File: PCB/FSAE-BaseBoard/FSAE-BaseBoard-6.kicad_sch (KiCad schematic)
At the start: 9 parts, among them J5 Conn_01x02, J6 Conn_01x03, J7 Conn_01x02, U9 SN65HVD230

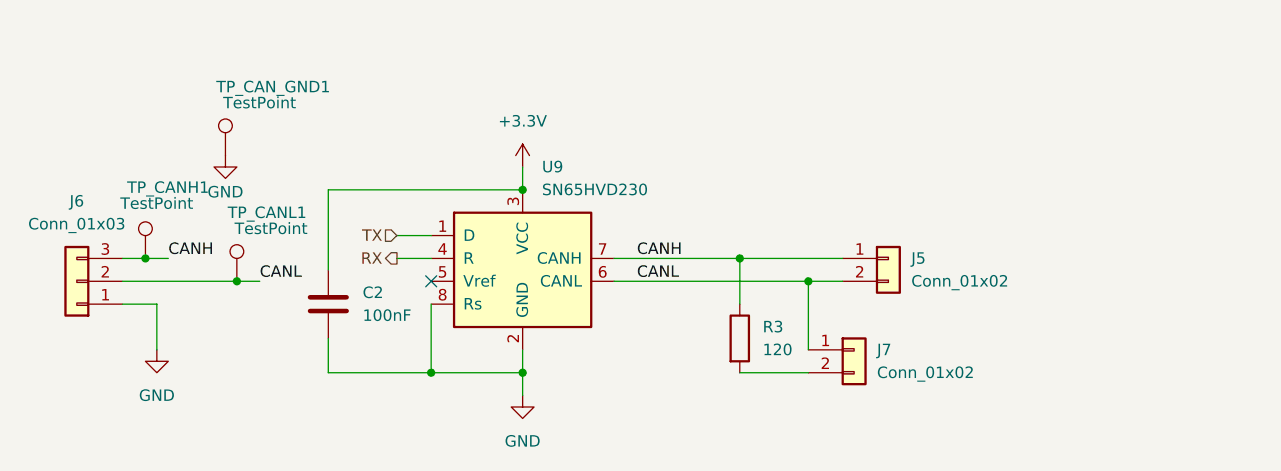
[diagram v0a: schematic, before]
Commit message: Actualizacion de la placa de desarollo - v.2
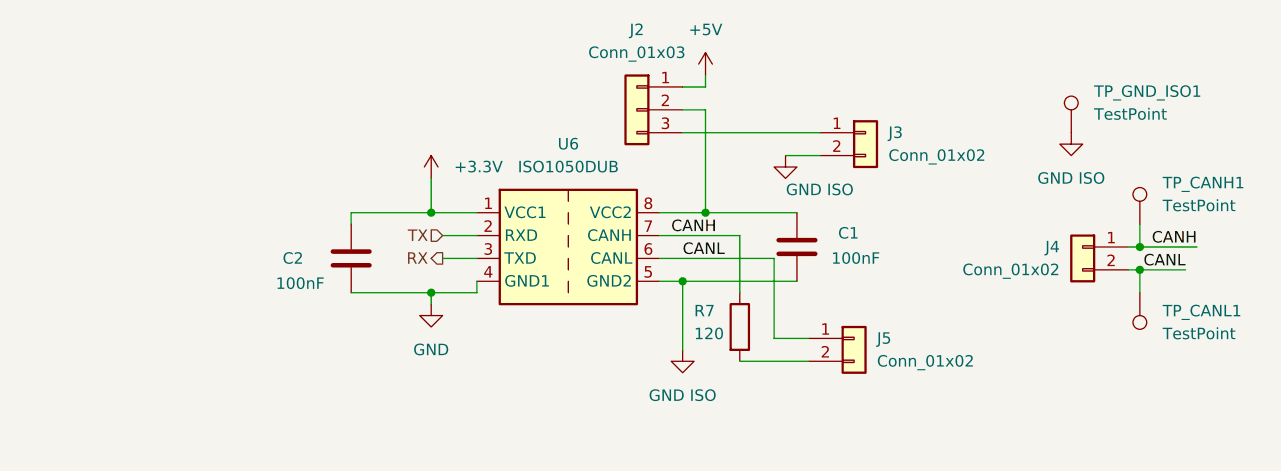
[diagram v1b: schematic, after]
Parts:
- removed J6: Conn_01x03, symbol Connector_Generic:Conn_01x03
- removed J7: Conn_01x02, symbol Connector_Generic:Conn_01x02
- removed R3: 120, symbol Device:R
- removed TP_CAN_GND1: TestPoint, symbol Connector:TestPoint
- removed U9: SN65HVD230, Package_SO:SOIC-8_3.9x4.9mm_P1.27mm, symbol Interface_CAN_LIN:SN65HVD230
- added C1: 100nF, symbol Device:C
- added J2: Conn_01x03, symbol Connector_Generic:Conn_01x03
- added J3, J4: Conn_01x02, symbol Connector_Generic:Conn_01x02
- added R7: 120, symbol Device:R
- added TP_GND_ISO1: TestPoint, symbol Connector:TestPoint
- added U6: ISO1050DUB, Package_SO:SOP-8_6.62x9.15mm_P2.54mm, symbol Interface_CAN_LIN:ISO1050DUB
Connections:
- net +3.3V: now also U6.1 (VCC1)
- net CANH: now also J4.1 (Pin_1), R7.1, U6.7 (CANH); no longer J5.1 (Pin_1)
- net CANL: now also J5.1 (Pin_1), J4.2 (Pin_2), U6.6 (CANL); no longer J5.2 (Pin_2)
- net GND: now also U6.4 (GND1)
- net RX: now also U6.3 (TXD)
- net TX: now also U6.2 (RXD)
- new net: C1.1, J2.2 (Pin_2), U6.8 (VCC2)
- new net: J2.3 (Pin_3), J3.1 (Pin_1)
- new net: J5.2 (Pin_2), R7.2
- new net +5V: J2.1 (Pin_1)
- new net GND ISO: C1.2, J3.2 (Pin_2), TP_GND_ISO1.1, U6.5 (GND2)
- no-connect marks 1 -> 0
